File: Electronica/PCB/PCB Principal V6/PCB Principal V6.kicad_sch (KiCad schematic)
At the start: 20 parts, among them J1 Conexion Sensores, J10 Conn_01x01, J2 Power Monster, J3 On/Off General, J4 Power Input 2, J5 IDC Placa Botones, J6 Power Input 1, J7 Conn_01x01, J8 Conn_01x01, J9 Conn_01x01, SW1 On/Off Motores

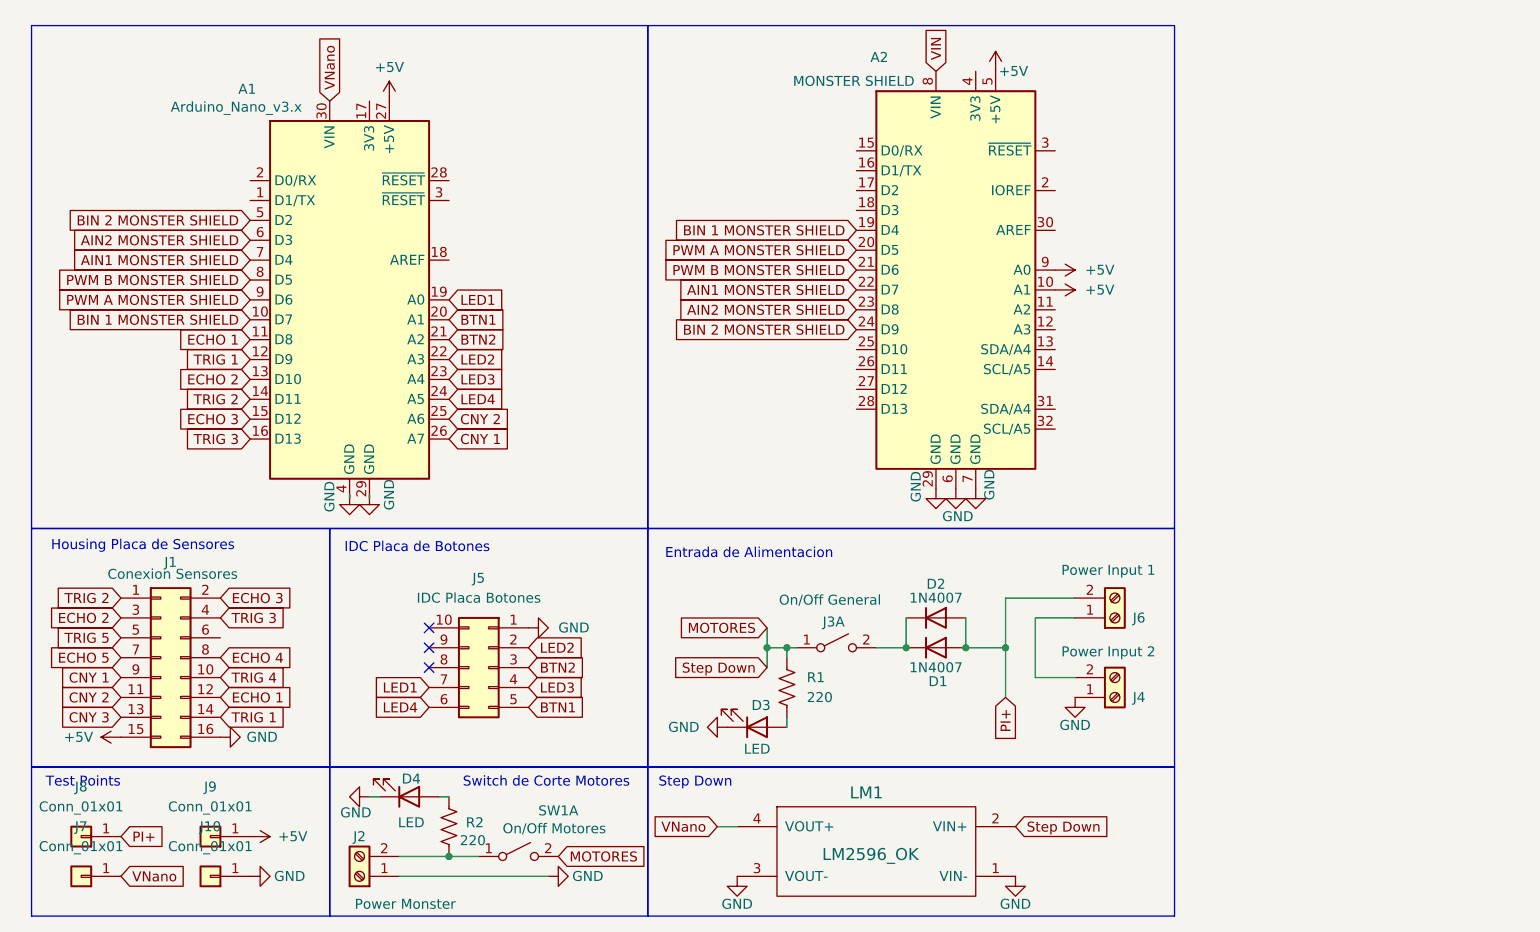
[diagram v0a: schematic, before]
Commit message: PCB V6 ACTUALIZADA
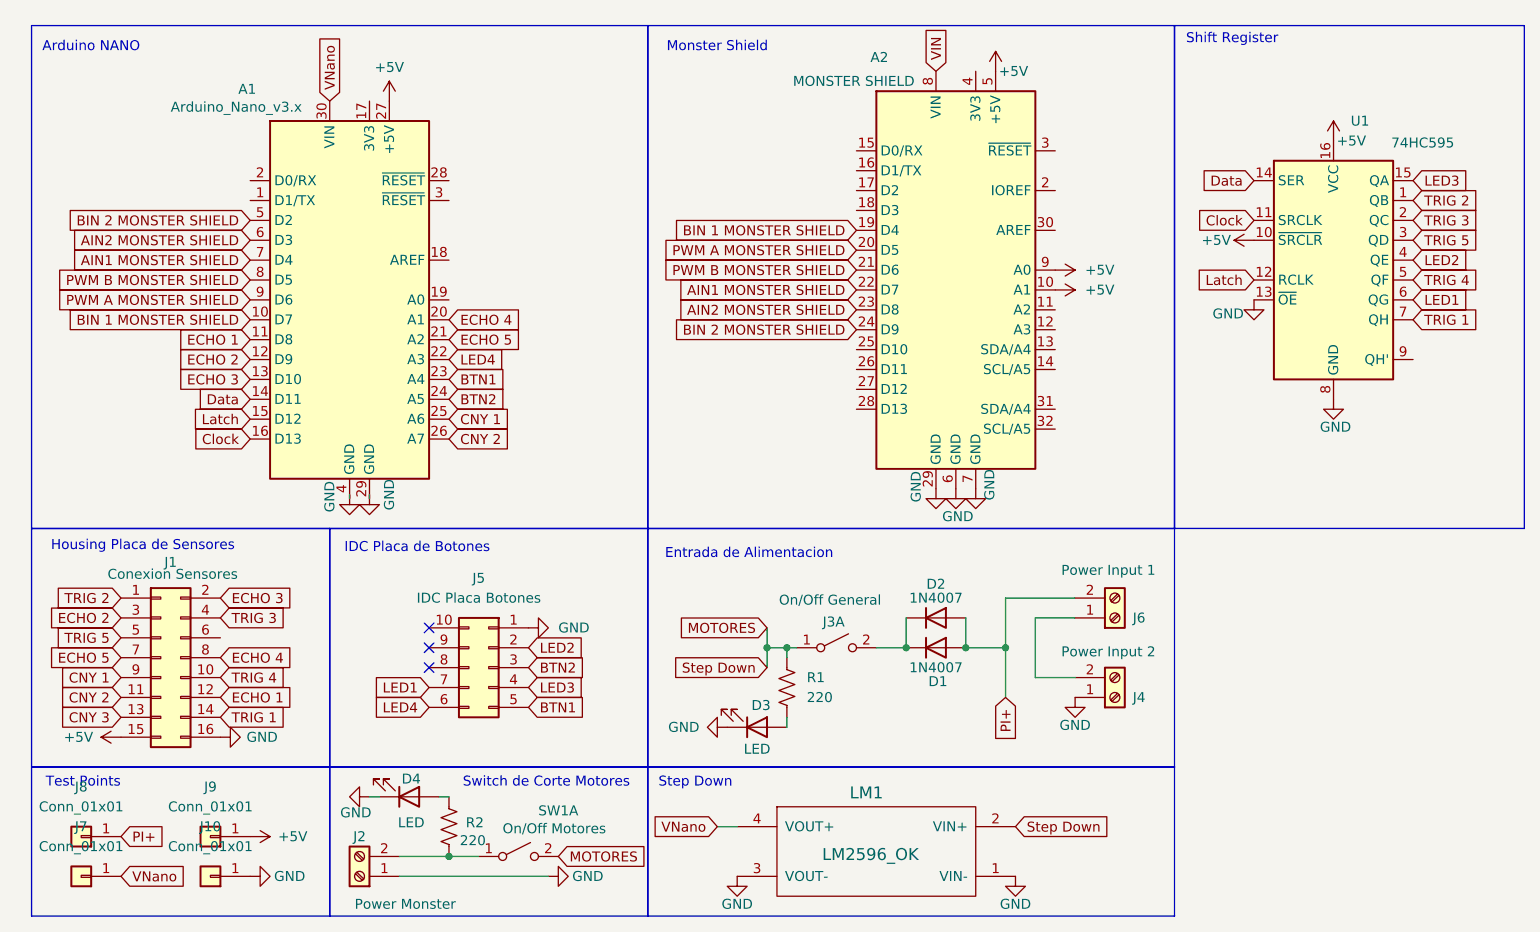
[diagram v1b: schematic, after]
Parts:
- added U1: 74HC595, 74HC595N_DIP16_:DIP16-2.54-20.32X5.84MM, symbol 74xx:74HC595
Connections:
- net +5V: now also U1.10 (~{SRCLR}), U1.16 (VCC)
- net BTN1: now also A1.23 (A4); no longer A1.20 (A1)
- net BTN2: now also A1.24 (A5); no longer A1.21 (A2)
- net CNY 1: now also A1.25 (A6); no longer A1.26 (A7)
- net CNY 2: now also A1.26 (A7); no longer A1.25 (A6)
- net ECHO 2: now also A1.12 (D9); no longer A1.13 (D10)
- net ECHO 3: now also A1.13 (D10); no longer A1.15 (D12)
- net ECHO 4: now also A1.20 (A1)
- net ECHO 5: now also A1.21 (A2)
- net GND: now also U1.13 (~{OE}), U1.8 (GND)
- net LED1: now also U1.6 (QG); no longer A1.19 (A0)
- net LED2: now also U1.4 (QE); no longer A1.22 (A3)
- net LED3: now also U1.15 (QA); no longer A1.23 (A4)
- net LED4: now also A1.22 (A3); no longer A1.24 (A5)
- net TRIG 1: now also U1.7 (QH); no longer A1.12 (D9)
- net TRIG 2: now also U1.1 (QB); no longer A1.14 (D11)
- net TRIG 3: now also U1.2 (QC); no longer A1.16 (D13)
- net TRIG 4: now also U1.5 (QF)
- net TRIG 5: now also U1.3 (QD)
- new net Clock: A1.16 (D13), U1.11 (SRCLK)
- new net Data: A1.14 (D11), U1.14 (SER)
- new net Latch: A1.15 (D12), U1.12 (RCLK)
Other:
- note added: "Arduino NANO"
- note added: "Monster Shield"
- note added: "Shift Register"
